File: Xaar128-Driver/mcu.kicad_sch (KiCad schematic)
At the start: 7 parts

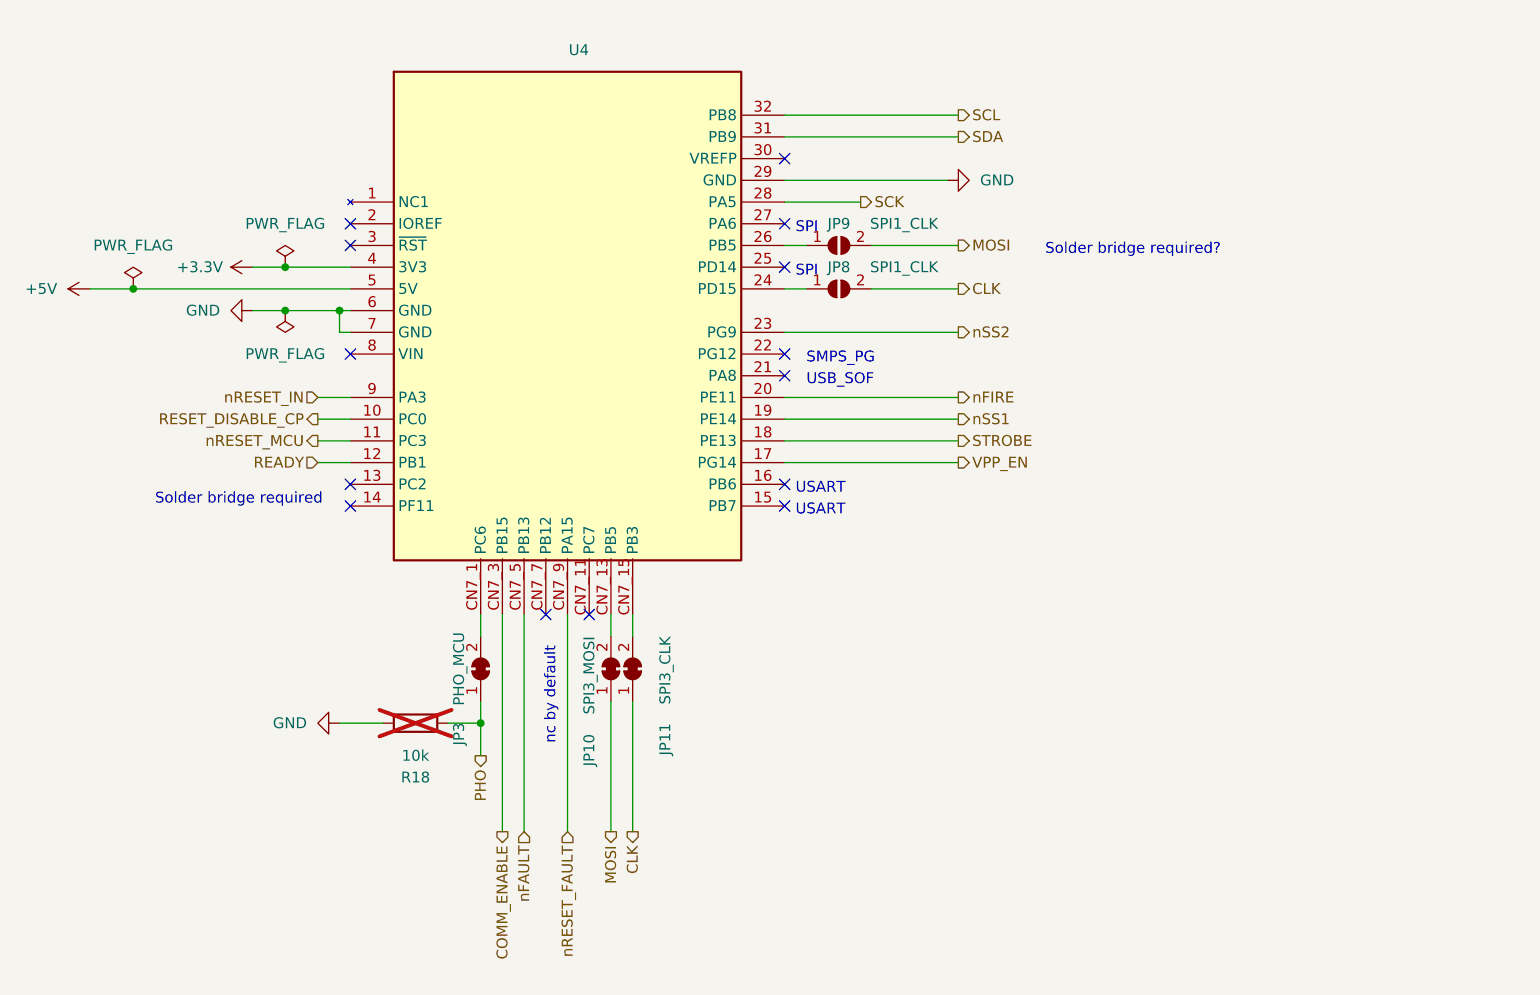
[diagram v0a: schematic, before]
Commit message: 5v monitoring
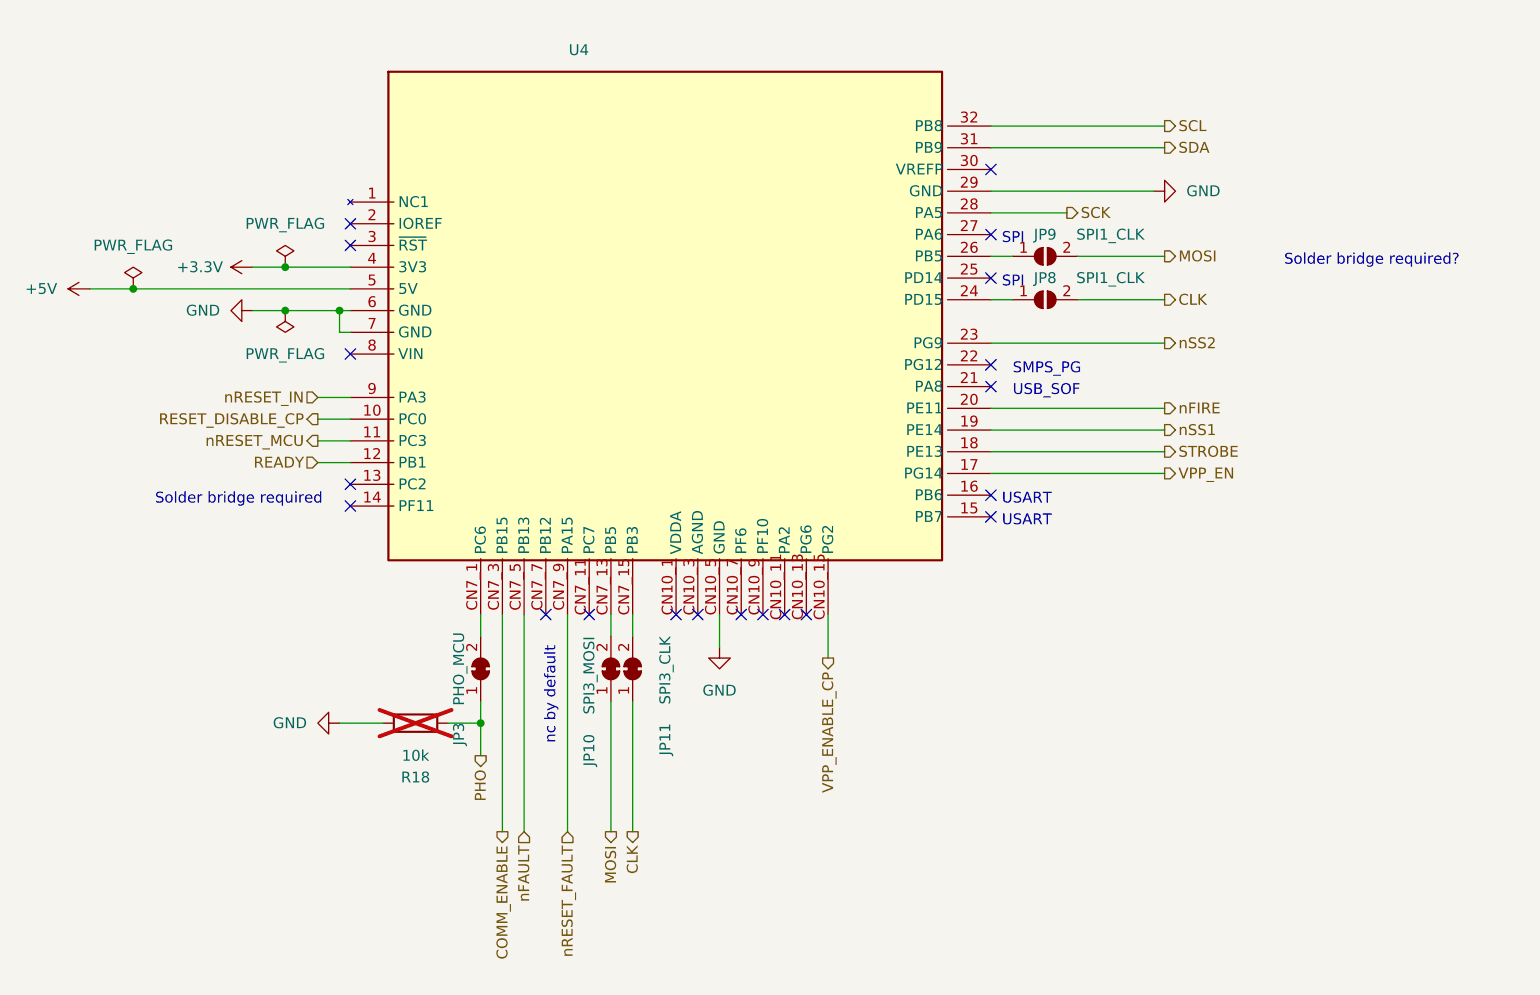
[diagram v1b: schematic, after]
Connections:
- net GND: now also U4.CN10_5 (GND)
- new net VPP_ENABLE_CP: U4.CN10_15 (PG2)
- no-connect marks 14 -> 20
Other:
- moved on the sheet: JP8, JP9

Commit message: some component selections, fix wrong mcu
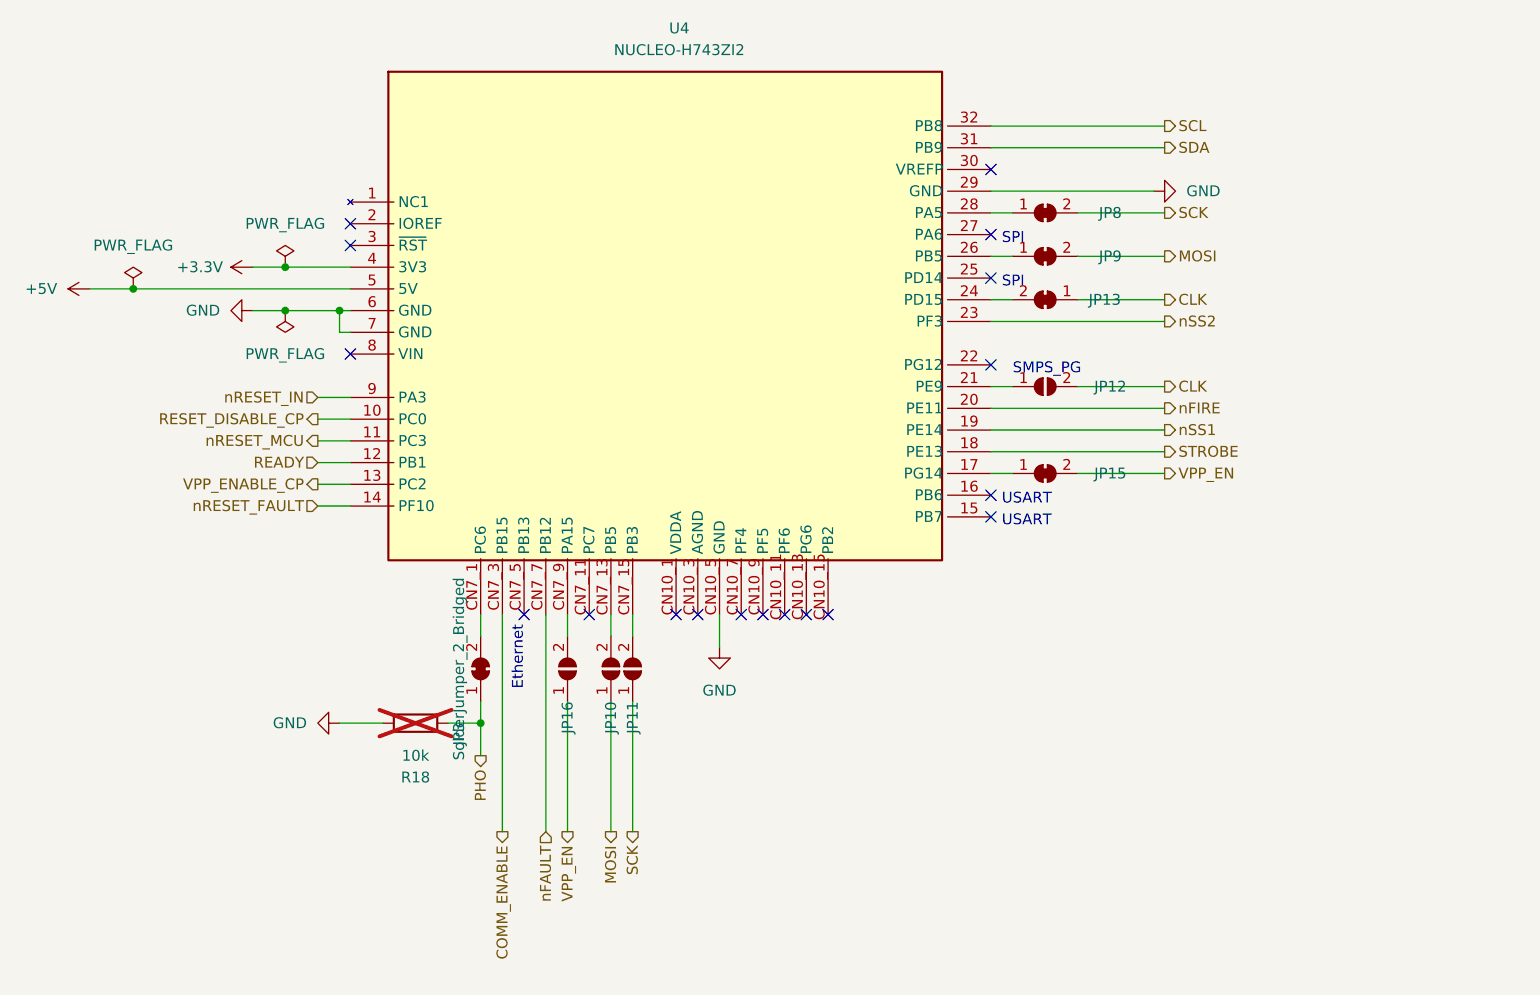
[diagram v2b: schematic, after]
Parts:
- removed JP8: SPI1_CLK, symbol Jumper:SolderJumper_2_Open
- added JP12, JP16: SolderJumper_2_Open, Resistor_SMD:R_0603_1608Metric, symbol Jumper:SolderJumper_2_Open
- added JP13, JP15, JP8: SolderJumper_2_Bridged, Resistor_SMD:R_0603_1608Metric, symbol Jumper:SolderJumper_2_Bridged
- JP10: value SPI3_MOSI -> SolderJumper_2_Open; footprint (none) -> Resistor_SMD:R_0603_1608Metric; symbol Jumper:SolderJumper_2_Bridged -> Jumper:SolderJumper_2_Open; Funktion (none) -> Connect MOSI to CN7; RSBestNr (none) -> 120-432; Supplier (none) -> RS
- JP11: value SPI3_CLK -> SolderJumper_2_Open; footprint (none) -> Resistor_SMD:R_0603_1608Metric; symbol Jumper:SolderJumper_2_Bridged -> Jumper:SolderJumper_2_Open; Funktion (none) -> Connect SCK to CN7; RSBestNr (none) -> 120-432; Supplier (none) -> RS
- JP3: value PHO_MCU -> SolderJumper_2_Bridged; footprint (none) -> Resistor_SMD:R_0603_1608Metric; Funktion (none) -> Disable MCU PHO Control; RSBestNr (none) -> 120-432; Supplier (none) -> RS
- JP9: value SPI1_CLK -> SolderJumper_2_Bridged; footprint (none) -> Resistor_SMD:R_0603_1608Metric; symbol Jumper:SolderJumper_2_Open -> Jumper:SolderJumper_2_Bridged; Funktion (none) -> Disconnes MOSI from Arduino; Supplier (none) -> None
- U4: value ~ -> NUCLEO-H743ZI2; symbol Xaar_Driver:NUCLEO-H745-Arduino -> Xaar_Driver:NUCLEO-H743-Arduino; RSBestNr (none) -> 193-9787; Supplier (none) -> RS
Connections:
- net CLK: now also JP12.2 (B), JP13.1 (A); no longer JP11.1 (A)
- net SCK: now also JP11.1 (A), JP8.2 (B); no longer U4.28 (PA5)
- net VPP_EN: now also JP15.2 (B), JP16.1 (A); no longer U4.17 (PG14)
- net VPP_ENABLE_CP: now also U4.13 (PC2); no longer U4.CN10_15 (PG2)
- net nFAULT: now also U4.CN7_7 (PB12); no longer U4.CN7_5 (PB13)
- net nRESET_FAULT: now also U4.14 (PF10); no longer U4.CN7_9 (PA15)
- net at U4.24 (PD15): now also JP13.2 (B)
- net at U4.21 (PE9): now also JP12.1 (A)
- new net: JP16.2 (B), U4.CN7_9 (PA15)
- new net: JP15.1 (A), U4.17 (PG14)
- new net: JP8.1 (A), U4.28 (PA5)
- no-connect marks 20 -> 18
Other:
- note added: "Ethernet"
- note removed: "Solder bridge required"
- note removed: "Solder bridge required?"
- note removed: "USB_SOF"
- note removed: "nc by default"

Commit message: assign footprints
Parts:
- R18: footprint (none) -> Resistor_SMD:R_0603_1608Metric_Pad0.98x0.95mm_HandSolder; Supplier (none) -> Elektroplatz
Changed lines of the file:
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@@
       (effects (font (size 1.27 1.27)))
     )
-    (property "Footprint" "" (at 124.46 121.412 90)
+    (property "Footprint" "Resistor_SMD:R_0603_1608Metric_Pad0.98x0.95mm_HandSolder" (at 124.46 121.412 90)
       (effects (font (size 1.27 1.27)) hide)
     )
@@
       (effects (font (size 1.27 1.27)) hide)
     )
-    (property "Supplier" "" (at 124.46 123.19 0)
+    (property "Supplier" "Elektroplatz" (at 124.46 123.19 0)
       (effects (font (size 1.27 1.27)) hide)
     )
